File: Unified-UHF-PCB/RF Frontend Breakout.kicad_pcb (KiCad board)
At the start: 2 copper layers, 82.5 x 82.5 mm, 74 parts, among them IC1 QPC1022SR, IC2 GRF5504, IC3 LHA-13LN+, IC4 QPC1022SR, J2 Conn_01x02, J3 Conn_01x02, J4 Conn_Coaxial, J5 Conn_01x05, J6 Conn_01x02, U1 AT86RF215-ZU, U3 NCS-62+, X1 TYETACSANF-26.000000

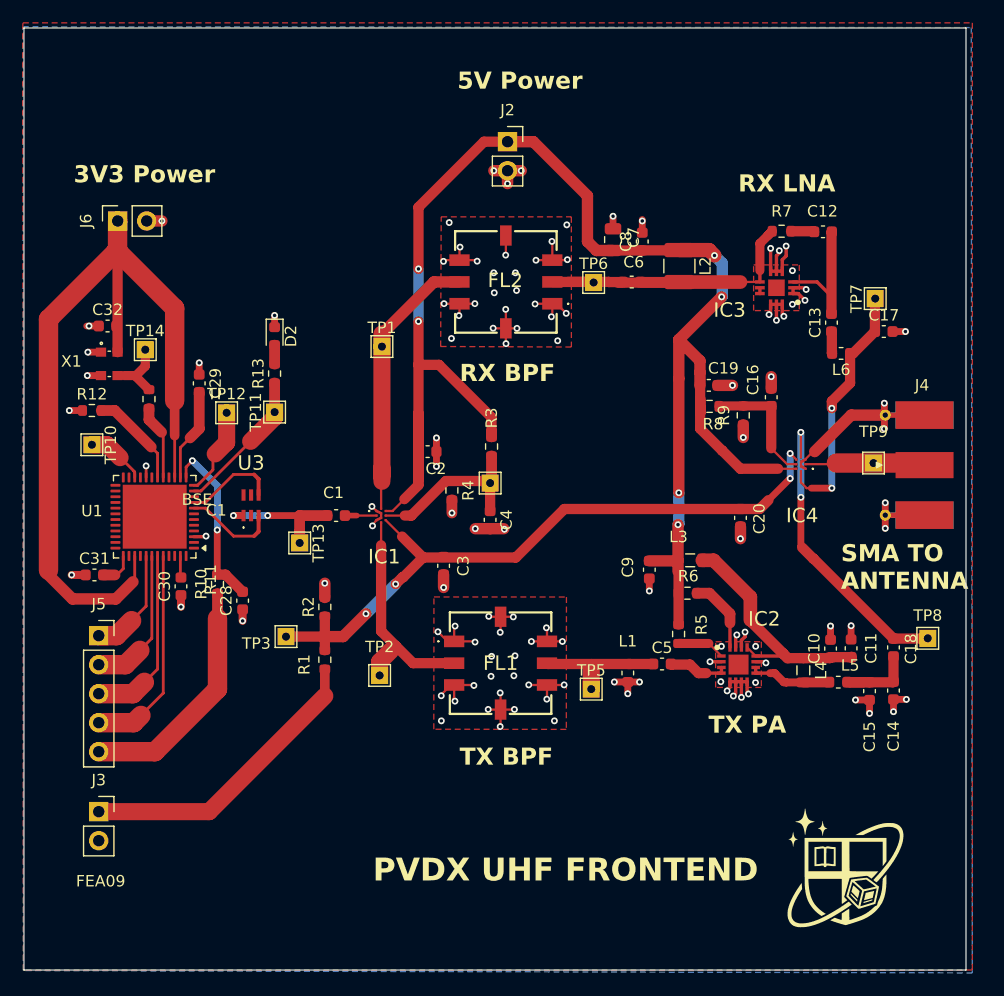
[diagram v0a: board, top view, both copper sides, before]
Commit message: saving first
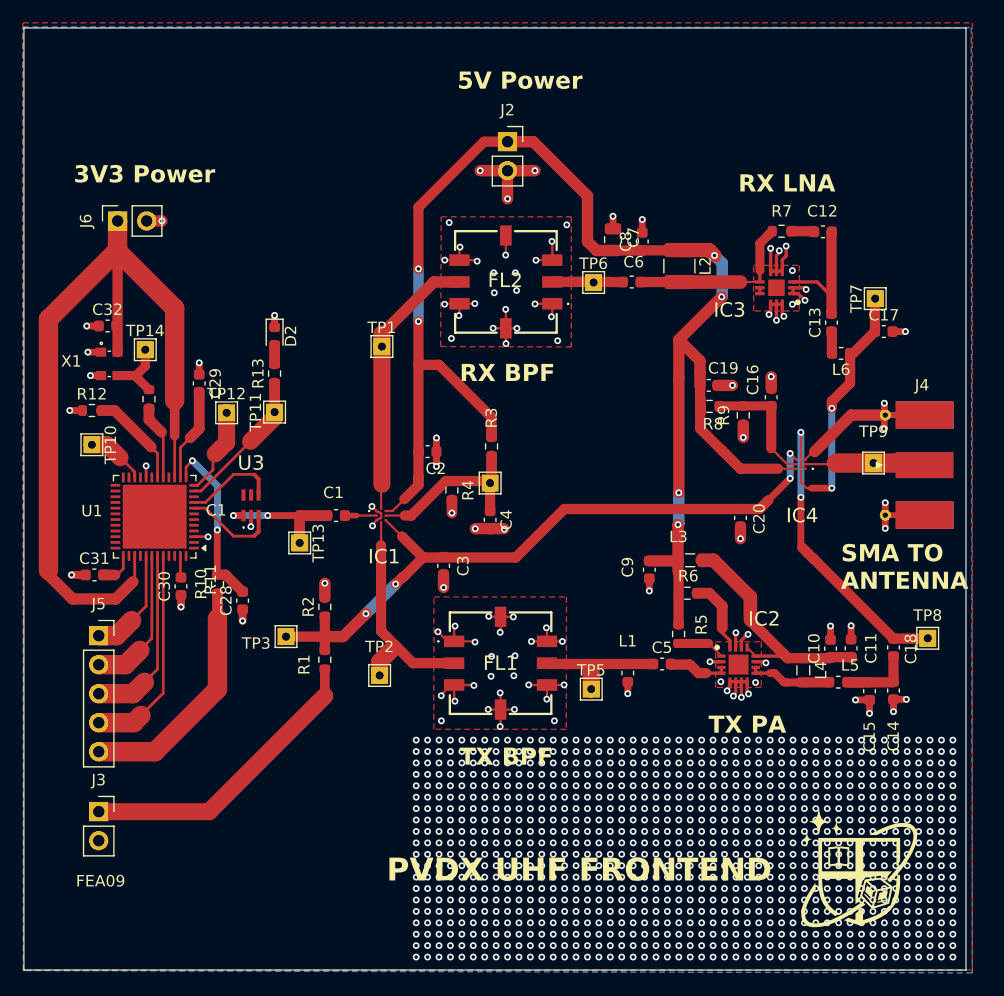
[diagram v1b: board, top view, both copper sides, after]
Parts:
- moved G*** 1.20 mm to (104.0, 91.9)
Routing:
- net +5V: track 138.7 -> 132.8 mm
- net Net-(FL2-RF_IN): track 13.4 -> 8.46 mm
- net Net-(IC4-RF1): track 27.5 -> 26.6 mm
- net Net-(FL2-RF_OUT): track 24.1 -> 23.5 mm
- net GND: track 133.7 -> 133.4 mm, vias 117 -> 1072

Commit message: small fixes
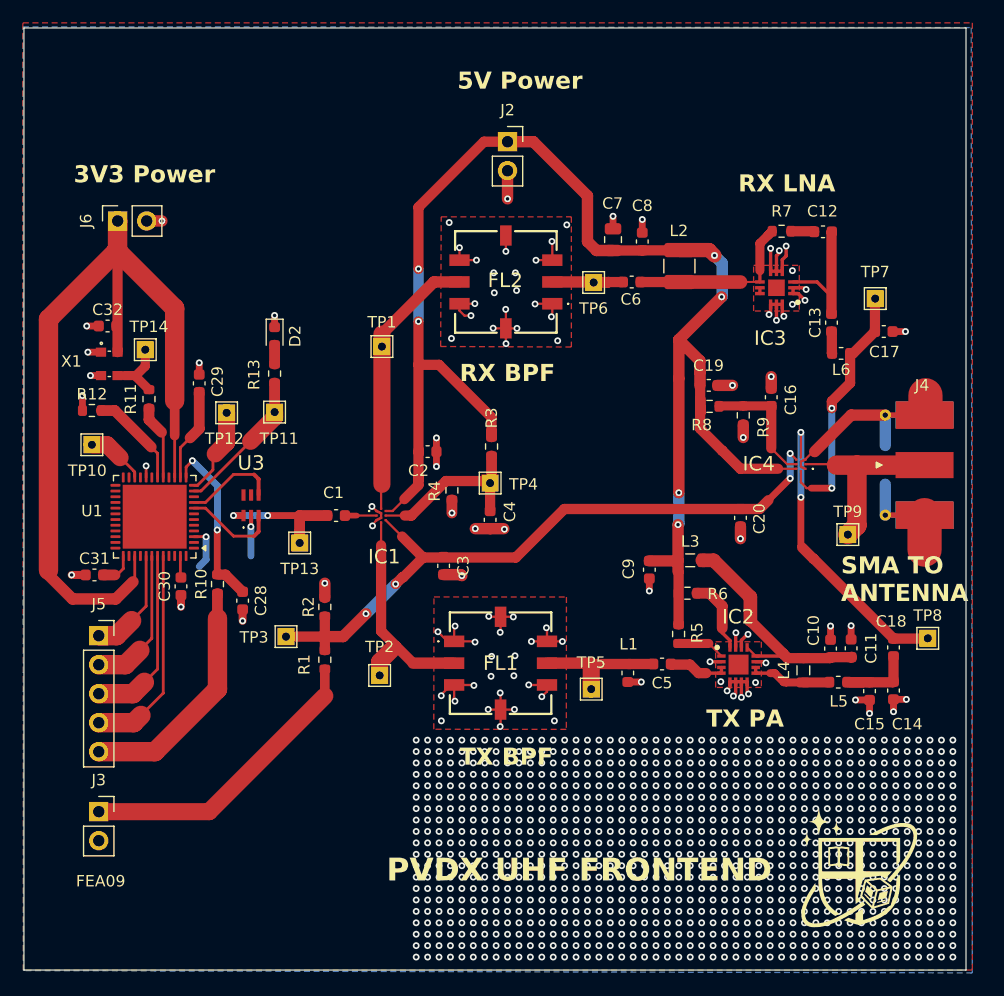
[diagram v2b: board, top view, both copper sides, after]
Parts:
- moved TP9 6.66 mm to (103.0, 62.4)
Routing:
- net Net-(IC4-ANT): track 11.1 -> 16.8 mm
- net GND: track 133.4 -> 136.2 mm, vias 1072 -> 1063
- net Net-(FL2-RF_IN): track 8.46 -> 7.55 mm
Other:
- board text added: "TP4"
- board text removed: "C1"
